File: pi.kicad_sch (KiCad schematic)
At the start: 3 parts, among them J33 2540-5

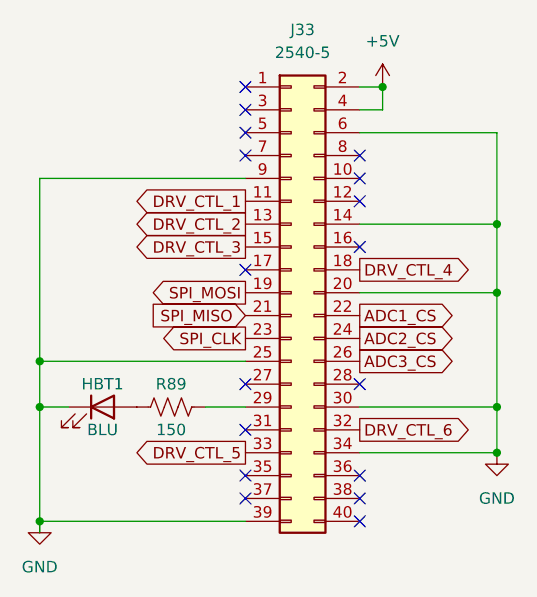
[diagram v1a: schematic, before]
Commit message: mostly finished routing
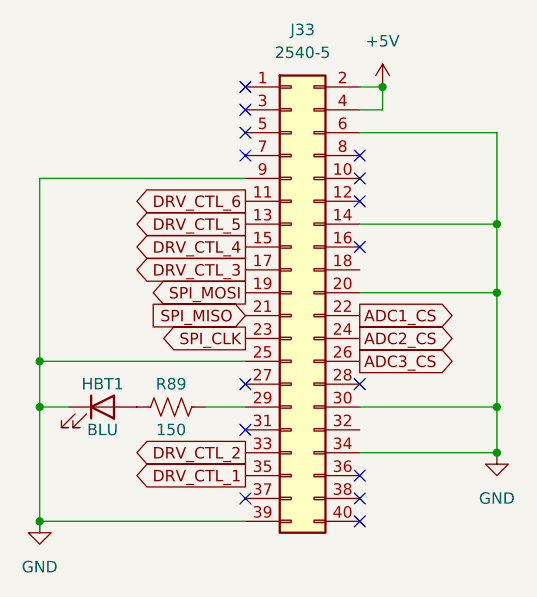
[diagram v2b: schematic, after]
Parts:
- J33: footprint Connector_PinHeader_2.54mm:PinHeader_2x20_P2.54mm_Horizontal -> Connector_PinSocket_2.54mm:PinSocket_2x20_P2.54mm_Horizontal
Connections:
- net DRV_CTL_1: now also J33.35 (Pin_35); no longer J33.11 (Pin_11)
- net DRV_CTL_2: now also J33.33 (Pin_33); no longer J33.13 (Pin_13)
- net DRV_CTL_3: now also J33.17 (Pin_17); no longer J33.15 (Pin_15)
- net DRV_CTL_4: now also J33.15 (Pin_15); no longer J33.18 (Pin_18)
- net DRV_CTL_5: now also J33.13 (Pin_13); no longer J33.33 (Pin_33)
- net DRV_CTL_6: now also J33.11 (Pin_11); no longer J33.32 (Pin_32)
- no-connect marks 17 -> 15
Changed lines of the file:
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@@
   (no_connect (at 111.76 110.49))
   (no_connect (at 99.06 95.25))
-  (no_connect (at 99.06 105.41))
   (no_connect (at 99.06 107.95))
-  (no_connect (at 99.06 82.55))
   (no_connect (at 99.06 100.33))
   (no_connect (at 111.76 95.25))
@@
     )
   )
-  (global_label "DRV_CTL_5" (shape output) (at 99.06 102.87 180) (fields_autoplaced)
+  (global_label "DRV_CTL_6" (shape output) (at 99.06 74.93 180) (fields_autoplaced)
+    (effects (font (size 1.27 1.27)) (justify right))
+    (property "Intersheet References" "${INTERSHEET_REFS}" (id 0) (at 86.6079 74.8506 0)
+      (effects (font (size 1.27 1.27)) (justify right) hide)
+    )
+  )
+  (global_label "DRV_CTL_2" (shape output) (at 99.06 102.87 180) (fields_autoplaced)
     (effects (font (size 1.27 1.27)) (justify right))
     (property "Intersheet References" "${INTERSHEET_REFS}" (id 0) (at 86.6079 102.7906 0)
@@
     )
   )
-  (global_label "DRV_CTL_3" (shape output) (at 99.06 80.01 180) (fields_autoplaced)
+  (global_label "DRV_CTL_1" (shape output) (at 99.06 105.41 180) (fields_autoplaced)
+    (effects (font (size 1.27 1.27)) (justify right))
+    (property "Intersheet References" "${INTERSHEET_REFS}" (id 0) (at 86.6079 105.3306 0)
+      (effects (font (size 1.27 1.27)) (justify right) hide)
+    )
+  )
+  (global_label "DRV_CTL_5" (shape output) (at 99.06 77.47 180) (fields_autoplaced)
+    (effects (font (size 1.27 1.27)) (justify right))
+    (property "Intersheet References" "${INTERSHEET_REFS}" (id 0) (at 86.6079 77.3906 0)
+      (effects (font (size 1.27 1.27)) (justify right) hide)
+    )
+  )
+  (global_label "DRV_CTL_4" (shape output) (at 99.06 80.01 180) (fields_autoplaced)
     (effects (font (size 1.27 1.27)) (justify right))
     (property "Intersheet References" "${INTERSHEET_REFS}" (id 0) (at 86.6079 79.9306 0)
-      (effects (font (size 1.27 1.27)) (justify right) hide)
-    )
-  )
-  (global_label "DRV_CTL_2" (shape output) (at 99.06 77.47 180) (fields_autoplaced)
-    (effects (font (size 1.27 1.27)) (justify right))
-    (property "Intersheet References" "${INTERSHEET_REFS}" (id 0) (at 86.6079 77.3906 0)
       (effects (font (size 1.27 1.27)) (justify right) hide)
     )
@@
     )
   )
-  (global_label "DRV_CTL_4" (shape output) (at 111.76 82.55 0) (fields_autoplaced)
-    (effects (font (size 1.27 1.27)) (justify left))
-    (property "Intersheet References" "${INTERSHEET_REFS}" (id 0) (at 124.2121 82.4706 0)
-      (effects (font (size 1.27 1.27)) (justify left) hide)
-    )
-  )
-  (global_label "DRV_CTL_1" (shape output) (at 99.06 74.93 180) (fields_autoplaced)
-    (effects (font (size 1.27 1.27)) (justify right))
-    (property "Intersheet References" "${INTERSHEET_REFS}" (id 0) (at 86.6079 74.8506 0)
-      (effects (font (size 1.27 1.27)) (justify right) hide)
-    )
-  )
   (global_label "SPI_CLK" (shape output) (at 99.06 90.17 180) (fields_autoplaced)
     (effects (font (size 1.27 1.27)) (justify right))
@@
     )
   )
-  (global_label "DRV_CTL_6" (shape output) (at 111.76 100.33 0) (fields_autoplaced)
-    (effects (font (size 1.27 1.27)) (justify left))
-    (property "Intersheet References" "${INTERSHEET_REFS}" (id 0) (at 124.2121 100.2506 0)
-      (effects (font (size 1.27 1.27)) (justify left) hide)
+  (global_label "DRV_CTL_3" (shape output) (at 99.06 82.55 180) (fields_autoplaced)
+    (effects (font (size 1.27 1.27)) (justify right))
+    (property "Intersheet References" "${INTERSHEET_REFS}" (id 0) (at 86.6079 82.4706 0)
+      (effects (font (size 1.27 1.27)) (justify right) hide)
     )
   )
@@
     (property "Reference" "J33" (id 0) (at 105.41 55.88 0))
     (property "Value" "2540-5" (id 1) (at 105.41 58.42 0))
-    (property "Footprint" "Connector_PinHeader_2.54mm:PinHeader_2x20_P2.54mm_Horizontal" (id 2) (at 104.14 85.09 0)
-      (effects (font (size 1.27 1.27)) hide)
-    )
+    (property "Footprint" "Connector_PinSocket_2.54mm:PinSocket_2x20_P2.54mm_Horizontal" (id 2) (at 104.14 85.09 0)
+      (effects (font (size 1.27 1.27)) hide)
+    )
